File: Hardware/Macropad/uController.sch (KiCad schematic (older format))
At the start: 17 parts, among them J1 Conn_02x03_Odd_Even, SW11 SW_Push, U1 ATmega32U4-AU, X1 KC2016K

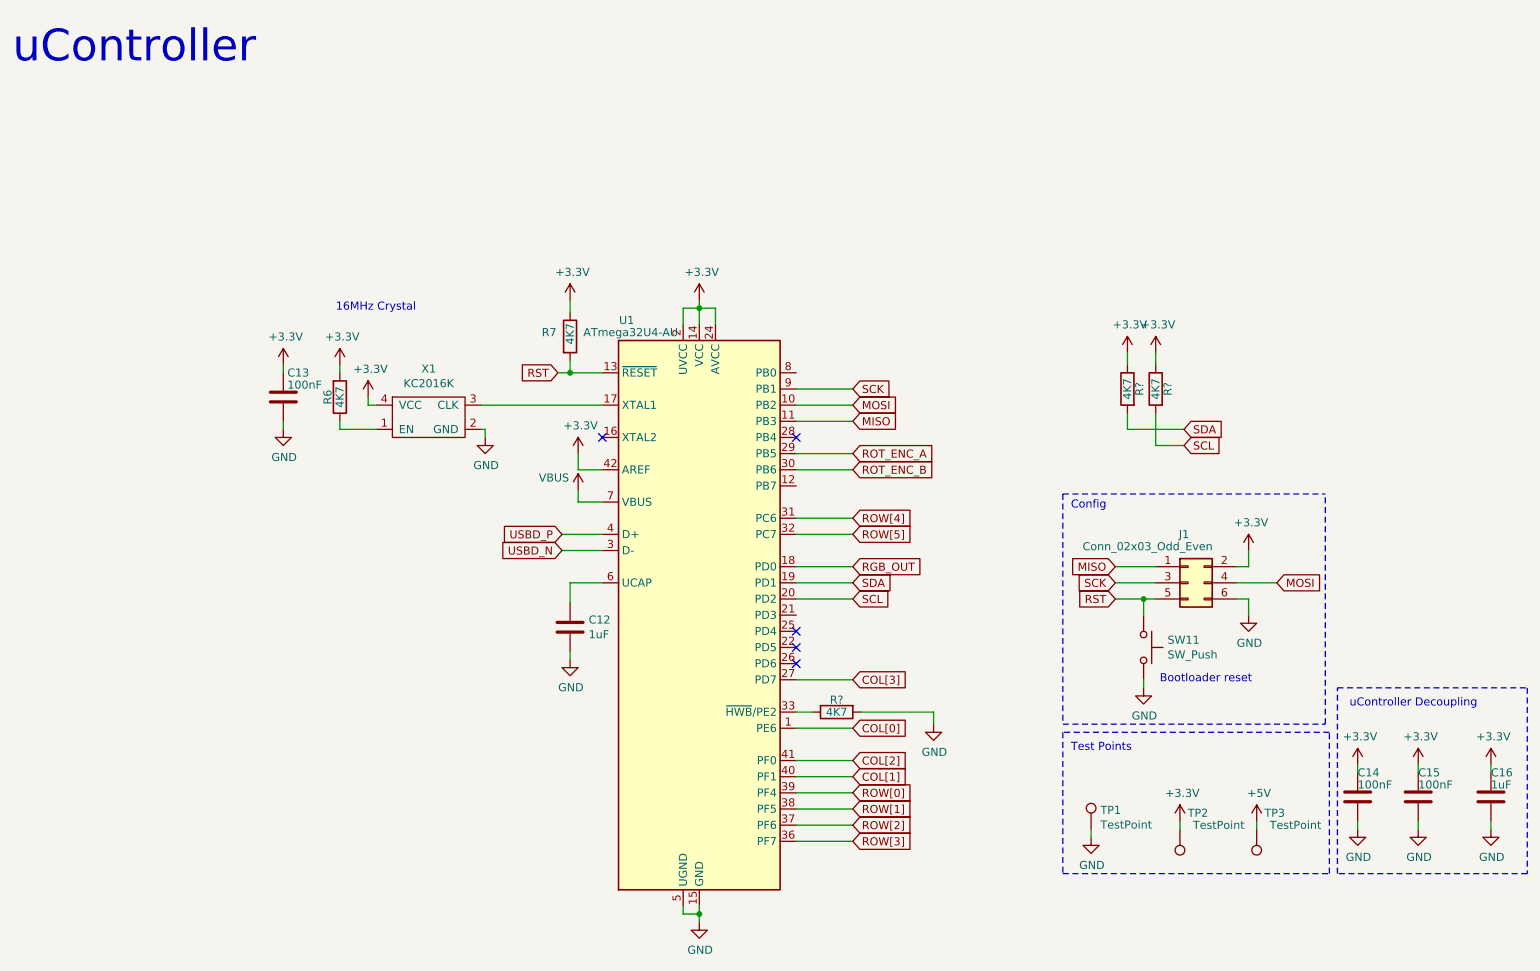
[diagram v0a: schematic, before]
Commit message: Schematic mostly done. Started grouping components in layout
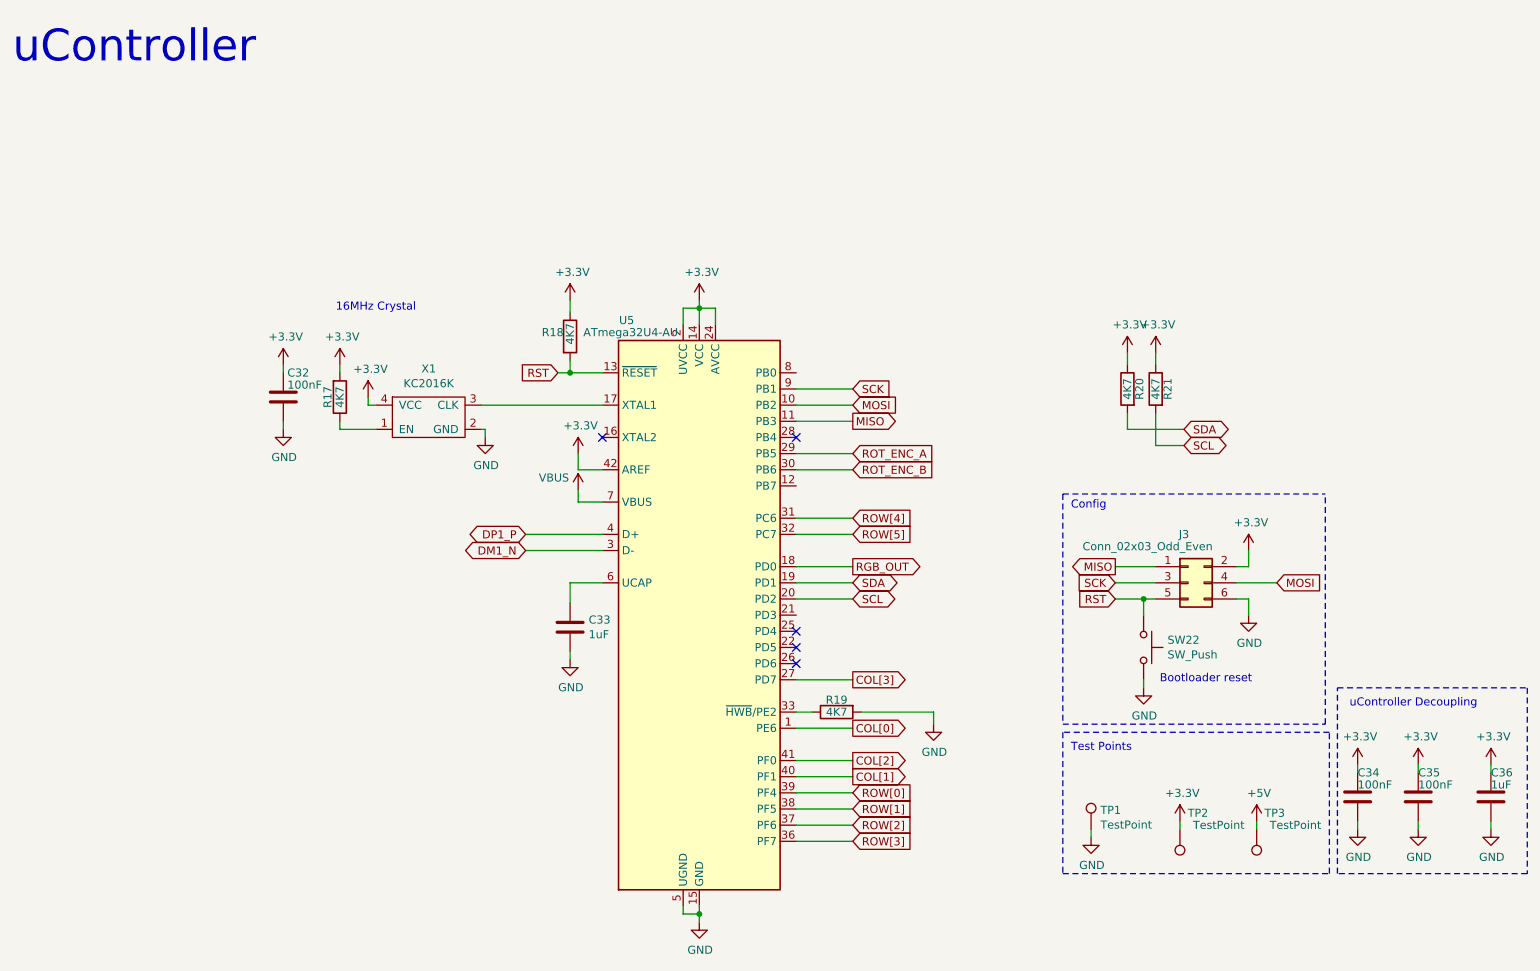
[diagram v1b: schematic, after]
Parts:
- gave numbers to parts that had none: 3
- renumbered C13 to C32, C12 to C33, C14 to C34, C15 to C35, C16 to C36, J1 to J3, R6 to R17, R7 to R18, SW11 to SW22, U1 to U5
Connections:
- net USBD_N renamed DM1_N
- net USBD_P renamed DP1_P

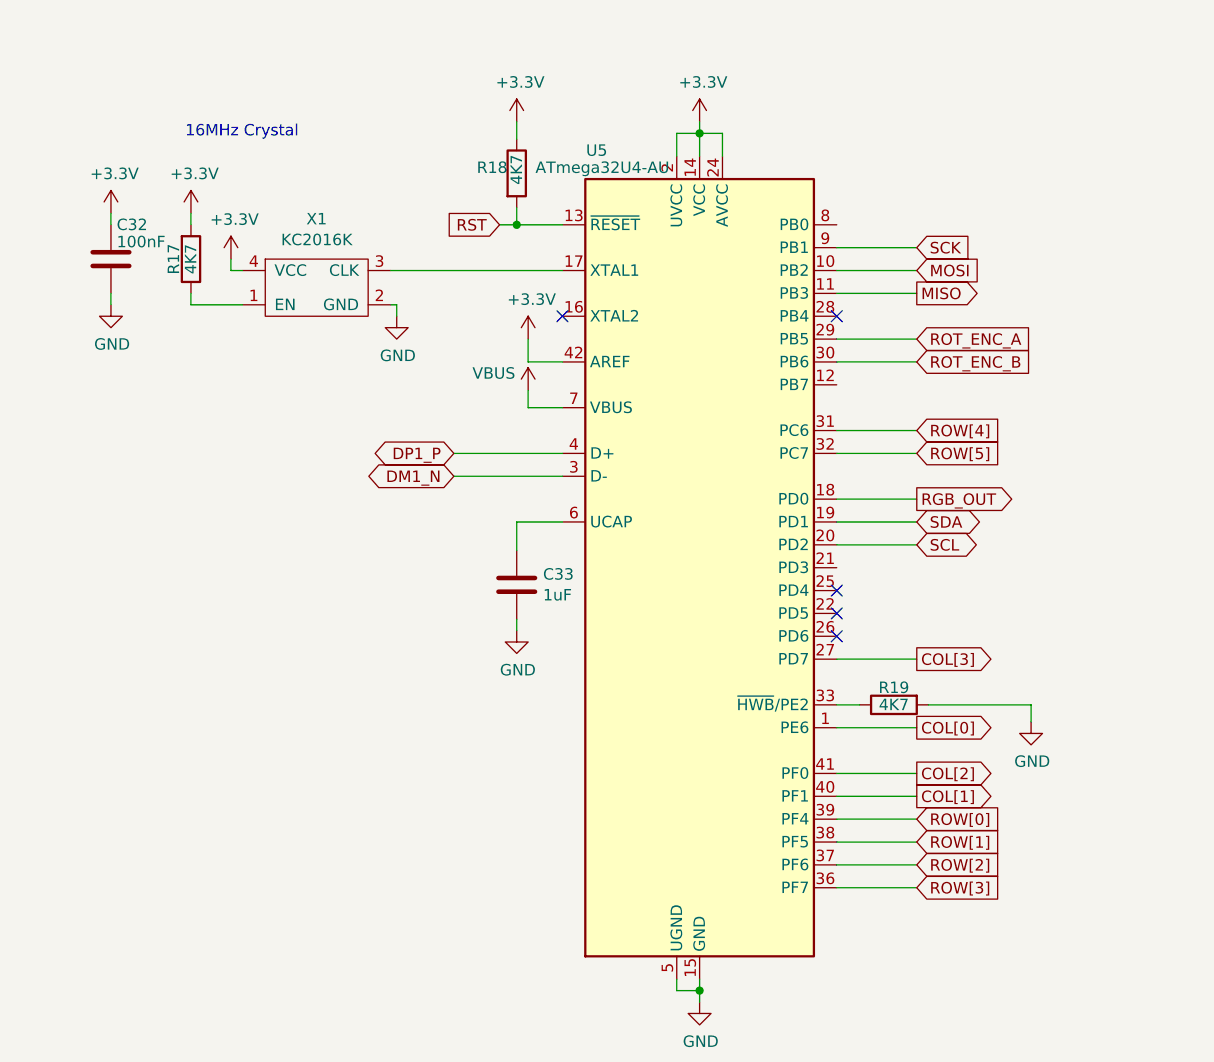
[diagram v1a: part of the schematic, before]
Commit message: First pass of the layout done
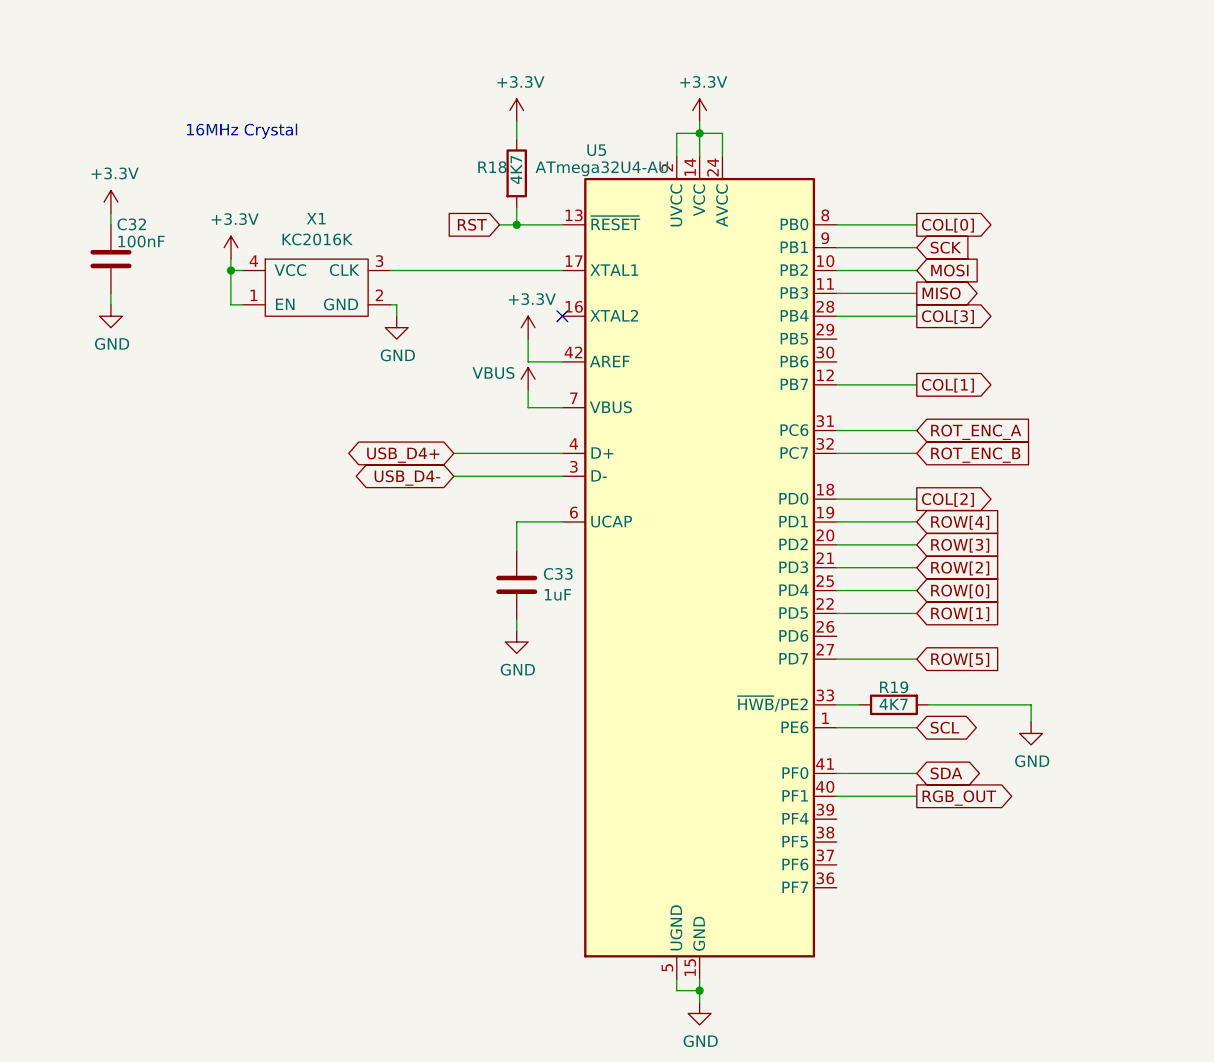
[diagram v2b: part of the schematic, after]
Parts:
- removed R17: 4K7, resistor_smd:R_0603_1608Metric, symbol Device:R
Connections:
- net +3V3: now also X1.1 (EN)
- net COL[0]: now also U5.8 (PB0); no longer U5.1 (PE6)
- net COL[1]: now also U5.12 (PB7); no longer U5.40 (PF1)
- net COL[2]: now also U5.18 (PD0); no longer U5.41 (PF0)
- net COL[3]: now also U5.28 (PB4); no longer U5.27 (PD7)
- net RGB_OUT: now also U5.40 (PF1); no longer U5.18 (PD0)
- net ROT_ENC_A: now also U5.31 (PC6); no longer U5.29 (PB5)
- net ROT_ENC_B: now also U5.32 (PC7); no longer U5.30 (PB6)
- net ROW[0]: now also U5.25 (PD4); no longer U5.39 (PF4)
- net ROW[1]: now also U5.22 (PD5); no longer U5.38 (PF5)
- net ROW[2]: now also U5.21 (PD3); no longer U5.37 (PF6)
- net ROW[3]: now also U5.20 (PD2); no longer U5.36 (PF7)
- net ROW[4]: now also U5.19 (PD1); no longer U5.31 (PC6)
- net ROW[5]: now also U5.27 (PD7); no longer U5.32 (PC7)
- net SCL: now also U5.1 (PE6); no longer U5.20 (PD2)
- net SDA: now also U5.41 (PF0); no longer U5.19 (PD1)
- net DM1_N renamed USB_D4-
- net DP1_P renamed USB_D4+
- no-connect marks 5 -> 1
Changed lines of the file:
@@
 Wire Wire Line
 	5000 6250 5000 6300
-Text GLabel 5950 5500 2    50   Input ~ 0
+Text GLabel 5950 4500 2    50   Input ~ 0
 ROW[0]
-Text GLabel 5950 5600 2    50   Input ~ 0
+Text GLabel 5950 4600 2    50   Input ~ 0
 ROW[1]
-Text GLabel 5950 5700 2    50   Input ~ 0
+Text GLabel 5950 4400 2    50   Input ~ 0
 ROW[2]
-Text GLabel 5950 5400 2    50   Output ~ 0
-COL[1]
-Text GLabel 5950 5300 2    50   Output ~ 0
-COL[2]
-Wire Wire Line
-	5600 5700 5950 5700
-Wire Wire Line
-	5600 5500 5950 5500
-Wire Wire Line
-	5600 5300 5950 5300
-Wire Wire Line
-	5600 5400 5950 5400
+Wire Wire Line
+	5600 4400 5950 4400
+Wire Wire Line
+	5600 4500 5950 4500
+Wire Wire Line
+	5600 4100 5950 4100
 $Comp
 L Device:C C?
@@
 Wire Wire Line
 	4200 2525 4200 2450
-Text GLabel 5950 3400 2    50   Input ~ 0
-ROT_ENC_A
-Text GLabel 5950 3500 2    50   Input ~ 0
-ROT_ENC_B
-Wire Wire Line
-	5600 3400 5950 3400
-Wire Wire Line
-	5600 3500 5950 3500
+Wire Wire Line
+	5600 3800 5950 3800
+Wire Wire Line
+	5600 3900 5950 3900
 Text Notes 750  1000 0    197  ~ 0
 uController
 NoConn ~ 4400 3300
-$Comp
-L Device:R R?
-U 1 1 60D6928E
-P 2775 3050
-AR Path="/60D6928E" Ref="R?"  Part="1"
-AR Path="/60D44BDB/60D6928E" Ref="R?"  Part="1"
-AR Path="/62022D96/60D6928E" Ref="R17"  Part="1"
-F 0 "R17" V 2700 3050 50  0000 C CNN
-F 1 "4K7" V 2775 3050 50  0000 C CNN
-F 2 "resistor_smd:R_0603_1608Metric" V 2705 3050 50  0001 C CNN
-F 3 "~" H 2775 3050 50  0001 C CNN
-	1    2775 3050
-	1    0    0    1
-$EndComp
 Wire Wire Line
 	2950 3100 2950 3050
 Wire Wire Line
 	3675 3300 3675 3250
-Wire Wire Line
-	2775 2850 2775 2900
 Wire Wire Line
 	3650 3100 4400 3100
@@
 Wire Notes Line
 	7250 3650 8875 3650
-Text GLabel 5950 5100 2    50   Output ~ 0
-COL[0]
-Wire Wire Line
-	5600 5600 5950 5600
+Wire Wire Line
+	5600 4600 5950 4600
 $Comp
 L power:VBUS #PWR?
@@
 	1    0    0    -1
 $EndComp
-NoConn ~ 5600 3300
-NoConn ~ 5600 4500
-NoConn ~ 5600 4600
-NoConn ~ 5600 4700
 Wire Wire Line
 	8400 4400 8400 4300
@@
 Wire Wire Line
 	4250 3400 4250 3500
-$Comp
-L power:+3.3V #PWR?
-U 1 1 60D692E9
-P 2775 2850
-AR Path="/60D692E9" Ref="#PWR?"  Part="1"
-AR Path="/60D44BDB/60D692E9" Ref="#PWR?"  Part="1"
-AR Path="/62022D96/60D692E9" Ref="#PWR0149"  Part="1"
-F 0 "#PWR0149" H 2775 2700 50  0001 C CNN
-F 1 "+3.3V" H 2790 3023 50  0000 C CNN
-F 2 "" H 2775 2850 50  0001 C CNN
-F 3 "" H 2775 2850 50  0001 C CNN
-	1    2775 2850
-	1    0    0    -1
-$EndComp
 $Comp
 L power:+3.3V #PWR?
@@
 	3650 3250 3675 3250
 Wire Wire Line
-	2775 3200 2775 3250
-Wire Wire Line
-	2775 3250 3000 3250
-Wire Wire Line
 	3000 3100 2950 3100
-Wire Wire Line
-	5950 5100 5600 5100
 $Comp
 L Switch:SW_Push SW22
@@
 Wire Notes Line
 	8875 5075 8875 3650
-Text GLabel 5950 3800 2    50   Input ~ 0
+Text GLabel 5950 4200 2    50   Input ~ 0
 ROW[4]
 Wire Wire Line
-	5950 3800 5600 3800
-Text GLabel 5950 4100 2    50   Output ~ 0
+	5950 4200 5600 4200
+Text GLabel 5950 5400 2    50   Output ~ 0
 RGB_OUT
 Wire Wire Line
-	5950 4100 5600 4100
+	5950 5400 5600 5400
 Text Notes 2750 2525 0    50   ~ 0
 16MHz Crystal
@@
 Wire Notes Line
 	10125 6000 8950 6000
-Text GLabel 5950 5800 2    50   Input ~ 0
+Text GLabel 5950 4300 2    50   Input ~ 0
 ROW[3]
 Wire Wire Line
-	5600 5800 5950 5800
+	5600 4300 5950 4300
 $Comp
 L Device:R R?
@@
 Wire Wire Line
 	6450 5000 6450 5075
-Text GLabel 5950 3900 2    50   Input ~ 0
+Text GLabel 5950 4800 2    50   Input ~ 0
 ROW[5]
 Wire Wire Line
-	5950 3900 5600 3900
-Text GLabel 5950 4800 2    50   Output ~ 0
-COL[3]
-Wire Wire Line
 	5950 4800 5600 4800
-Text GLabel 5950 4200 2    50   BiDi ~ 0
+Wire Wire Line
+	5950 3300 5600 3300
+Text GLabel 5950 5300 2    50   BiDi ~ 0
 SDA
 Wire Wire Line
-	5950 4200 5600 4200
-Text GLabel 5950 4300 2    50   BiDi ~ 0
+	5950 5300 5600 5300
+Text GLabel 5950 5100 2    50   BiDi ~ 0
 SCL
 Wire Wire Line
-	5950 4300 5600 4300
+	5950 5100 5600 5100
 $Comp
 L Device:R R?
@@
 Wire Wire Line
 	3925 4000 4400 4000
-Text GLabel 3925 3900 0    50   BiDi ~ 0
-DP1_P
-Text GLabel 3925 4000 0    50   BiDi ~ 0
-DM1_N
 Text GLabel 8000 3250 2    50   BiDi ~ 0
 SDA
+Wire Wire Line
+	3000 3250 2950 3250
+Wire Wire Line
+	2950 3250 2950 3100
+Connection ~ 2950 3100
+Wire Wire Line
+	5600 3600 5950 3600
+Text GLabel 5950 4100 2    50   Output ~ 0
+COL[2]
+Wire Wire Line
+	5950 2900 5600 2900
+Text GLabel 5950 2900 2    50   Output ~ 0
+COL[0]
+Text GLabel 5950 3600 2    50   Output ~ 0
+COL[1]
+Text GLabel 5950 3900 2    50   Input ~ 0
+ROT_ENC_B
+Text GLabel 5950 3800 2    50   Input ~ 0
+ROT_ENC_A
+Text GLabel 5950 3300 2    50   Output ~ 0
+COL[3]
+Text GLabel 3925 3900 0    50   BiDi ~ 0
+USB_D4+
+Text GLabel 3925 4000 0    50   BiDi ~ 0
+USB_D4-
 $EndSCHEMATC
